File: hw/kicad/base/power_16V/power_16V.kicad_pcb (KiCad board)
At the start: 2 copper layers, 45 x 45 mm, 38 parts, among them J1 USB_B_Micro, J3 TOP, J4 BUTTOM, U1 LM2596S-5, U2 LM1117MP-3.3, U3 CP2104, U4 ACS712xLCTR-05B

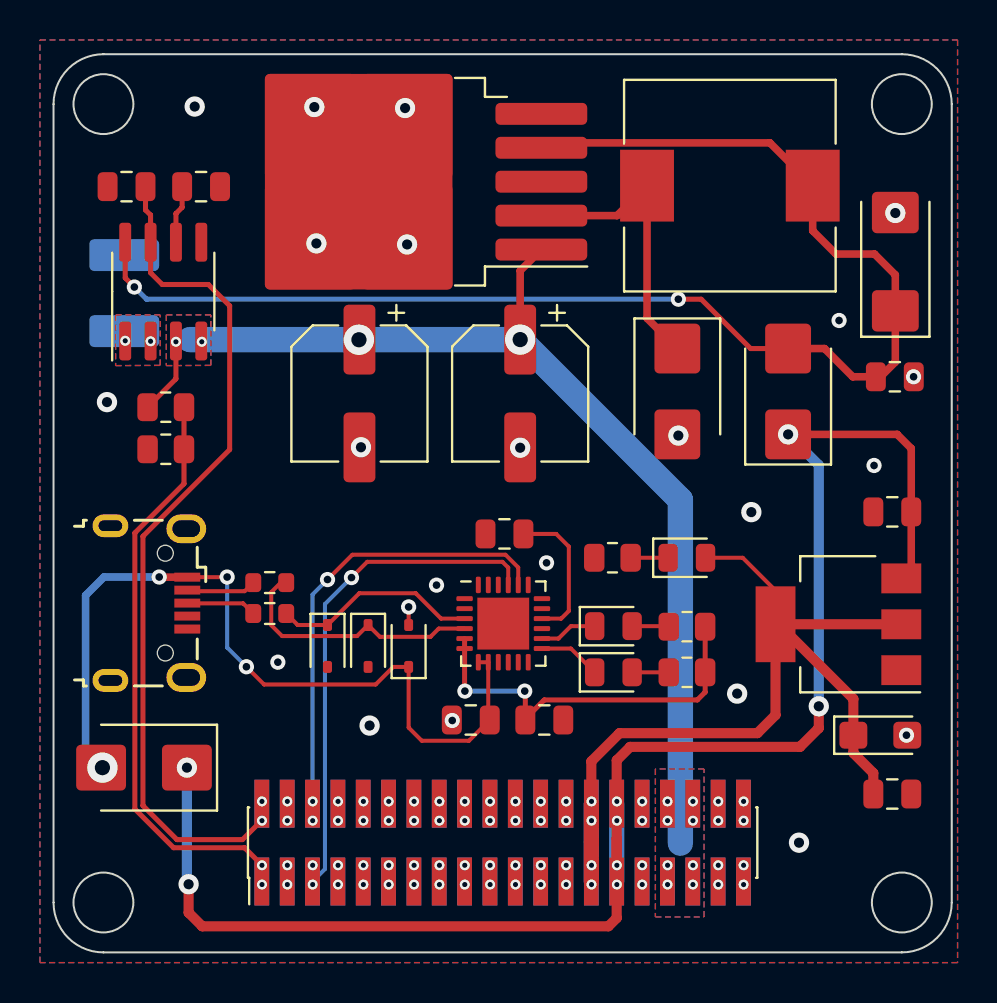
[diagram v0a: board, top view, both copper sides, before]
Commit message: 更新CPU板
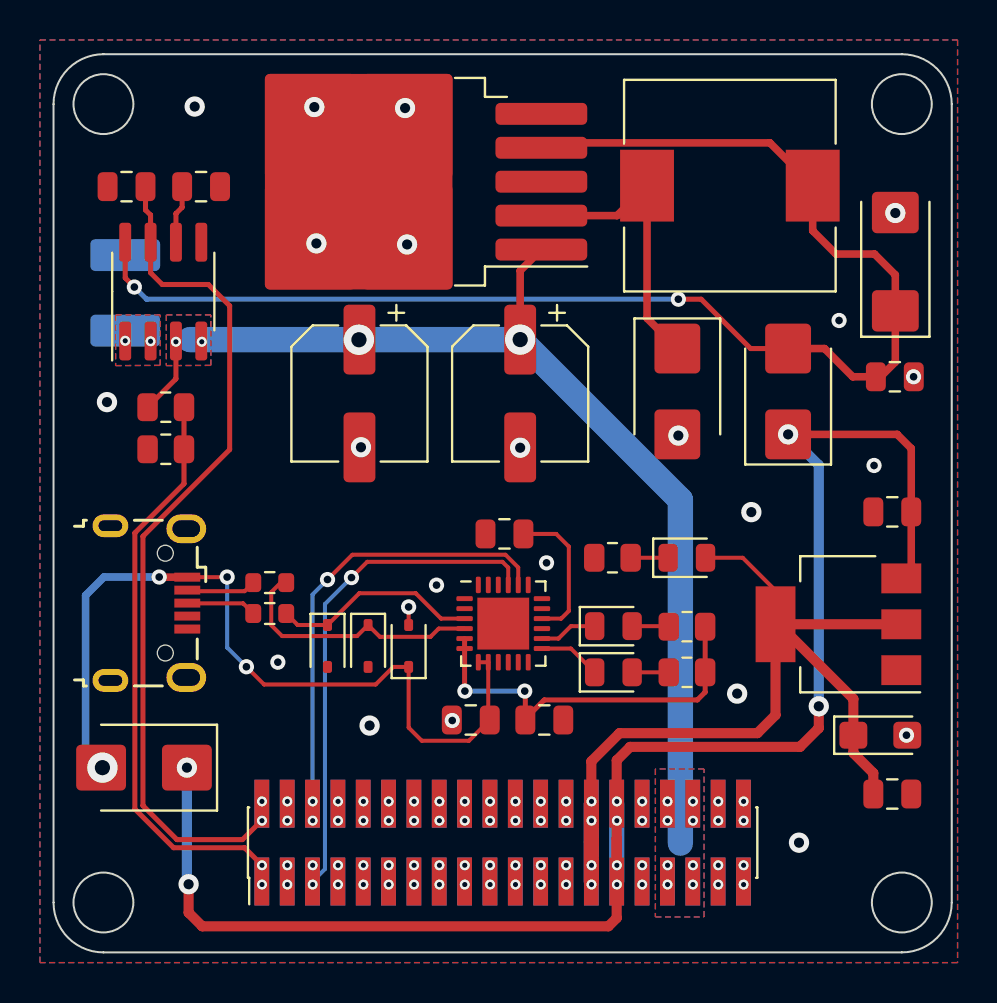
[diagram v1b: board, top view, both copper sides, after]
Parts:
- moved ? 0.06 mm to (54.3, 46.6)
- moved ? 0.05 mm to (54.3, 42.8)
